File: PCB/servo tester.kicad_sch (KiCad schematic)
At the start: 5 parts, among them U1 ER_OLEDM0.91_1x-I2C

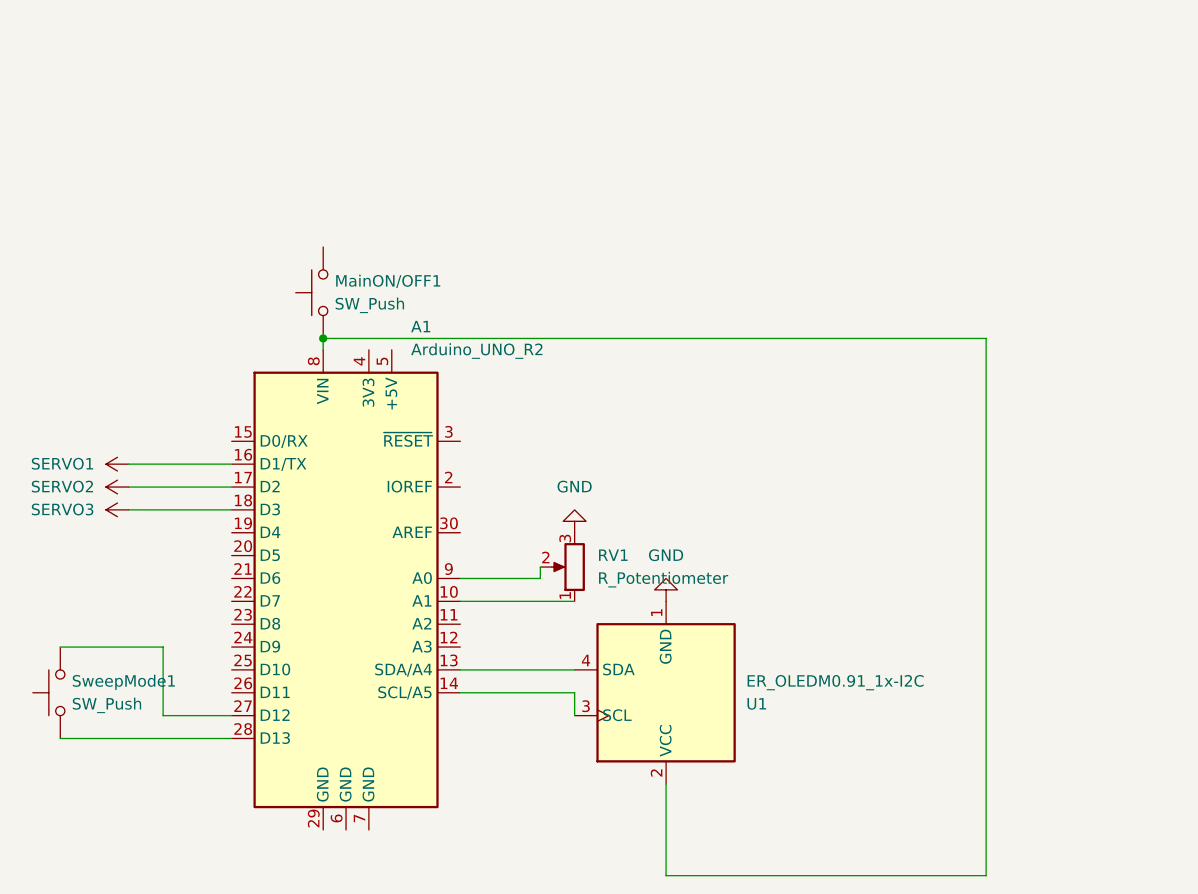
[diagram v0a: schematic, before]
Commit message: done a quite a bit of PCB
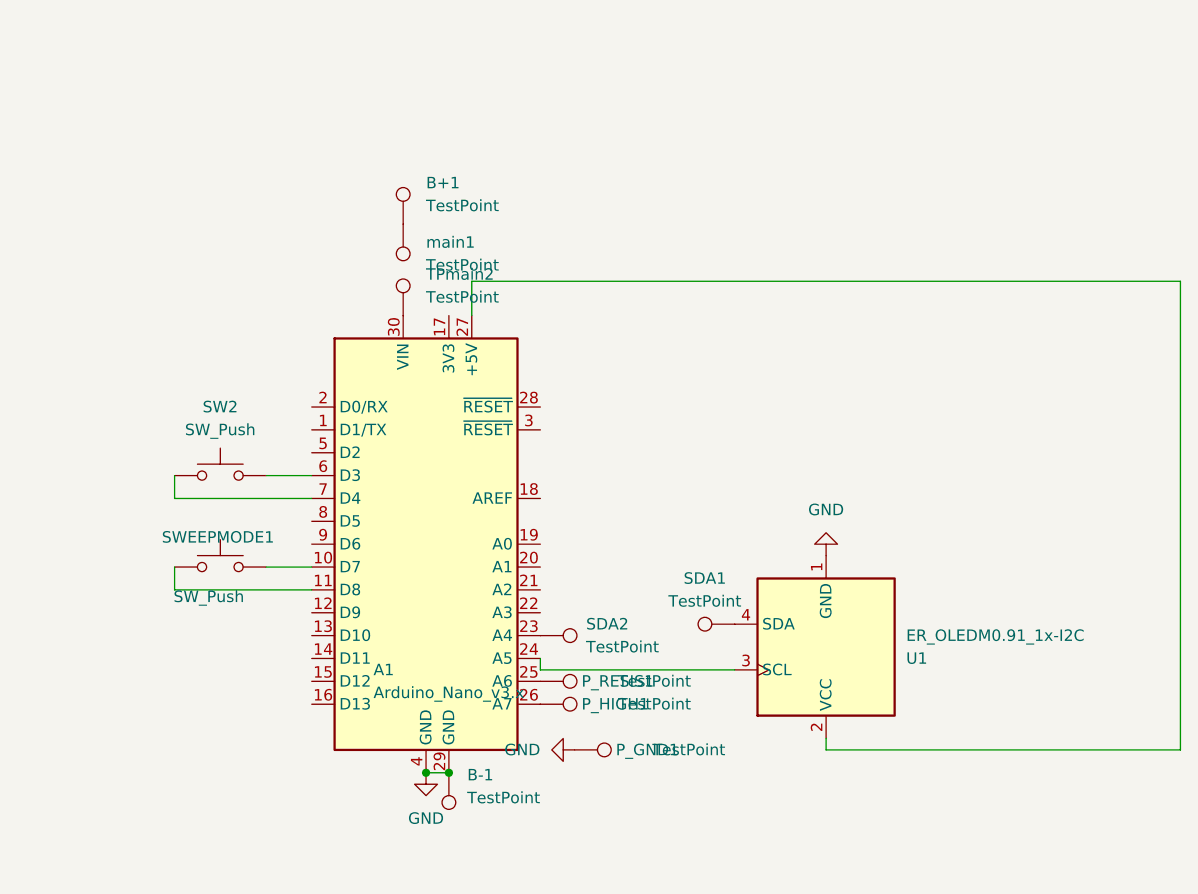
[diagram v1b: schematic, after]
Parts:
- removed A1: Arduino_UNO_R2, Module:Arduino_UNO_R2, symbol MCU_Module:Arduino_UNO_R2
- removed MainON/OFF1, SweepMode1: SW_Push, Button_Switch_THT:SW_PUSH_6mm_H13mm, symbol Switch:SW_Push
- removed RV1: R_Potentiometer, symbol Device:R_Potentiometer
- added A1: Arduino_Nano_v3.x, Module:Arduino_Nano, symbol MCU_Module:Arduino_Nano_v3.x
- added B+1, B-1, P_GND1, P_HIGH1, P_RESIS1, SDA1, SDA2, TPmain2, main1: TestPoint, Connector_Wire:SolderWire-0.75sqmm_1x01_D1.25mm_OD2.3mm, symbol Connector:TestPoint
- added SW2, SWEEPMODE1: SW_Push, Button_Switch_THT:SW_PUSH_6mm_H4.3mm, symbol Switch:SW_Push
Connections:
- net GND: now also A1.29 (GND), A1.4 (GND), B-1.1, P_GND1.1
- net at U1.2 (VCC): now also A1.27 (+5V)
- net at U1.3 (SCL): now also A1.24 (A5)
- net at U1.4 (SDA): now also SDA1.1
- new net: A1.10 (D7), SWEEPMODE1.2
- new net: A1.11 (D8), SWEEPMODE1.1
- new net: A1.23 (A4), SDA2.1
- new net: A1.25 (A6), P_RESIS1.1
- new net: A1.26 (A7), P_HIGH1.1
- new net: A1.30 (VIN), TPmain2.1
- new net: A1.6 (D3), SW2.2
- new net: A1.7 (D4), SW2.1
- new net: B+1.1, main1.1

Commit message: redid pcb
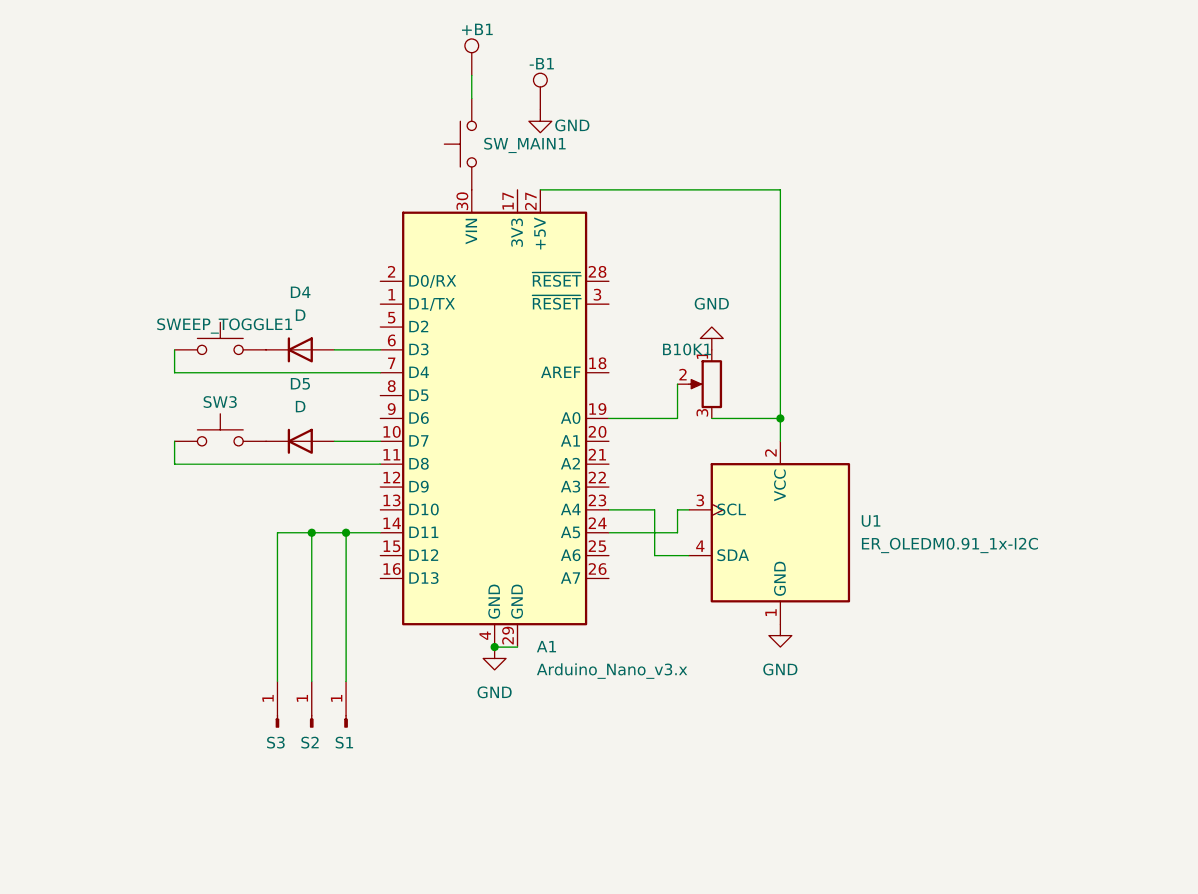
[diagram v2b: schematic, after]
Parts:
- removed B+1, B-1, P_GND1, P_HIGH1, P_RESIS1, SDA1, SDA2, TPmain2, main1: TestPoint, Connector_Wire:SolderWire-0.75sqmm_1x01_D1.25mm_OD2.3mm, symbol Connector:TestPoint
- removed SW2, SWEEPMODE1: SW_Push, Button_Switch_THT:SW_PUSH_6mm_H4.3mm, symbol Switch:SW_Push
- added +B1, -B1: TestPoint, Connector_Wire:SolderWire-0.5sqmm_1x01_D0.9mm_OD2.1mm, symbol Connector:TestPoint
- added B10K1: R_Potentiometer, Potentiometer_THT:Potentiometer_Bourns_3386C_Horizontal, symbol Device:R_Potentiometer
- added D4, D5: D, Diode_THT:D_A-405_P10.16mm_Horizontal, symbol Device:D
- added S1, S2, S3: Conn_01x01_Pin, Connector_PinHeader_2.54mm:PinHeader_1x01_P2.54mm_Horizontal, symbol Connector:Conn_01x01_Pin
- added SW3, SWEEP_TOGGLE1: SW_Push, Button_Switch_THT:SW_PUSH_6mm, symbol Switch:SW_Push
- added SW_MAIN1: SW_Push, Button_Switch_THT:SW_DIP_SPSTx01_Slide_9.78x4.72mm_W7.62mm_P2.54mm, symbol Switch:SW_Push
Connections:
- net GND: now also -B1.1, B10K1.1
- net at A1.10 (D7): now also D5.2 (A)
- net at A1.11 (D8): now also SW3.1
- net at A1.14 (D11): now also S1.1 (Pin_1), S2.1 (Pin_1), S3.1 (Pin_1)
- net at A1.19 (A0): now also B10K1.2
- net at A1.23 (A4): now also U1.4 (SDA)
- net at A1.27 (+5V), U1.2 (VCC): now also B10K1.3
- net at A1.30 (VIN): now also SW_MAIN1.1
- net at A1.6 (D3): now also D4.2 (A)
- net at A1.7 (D4): now also SWEEP_TOGGLE1.1
- new net: +B1.1, SW_MAIN1.2
- new net: D5.1 (K), SW3.2
- new net: D4.1 (K), SWEEP_TOGGLE1.2
